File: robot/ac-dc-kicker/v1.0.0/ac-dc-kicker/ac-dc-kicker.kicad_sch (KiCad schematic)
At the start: 9 parts

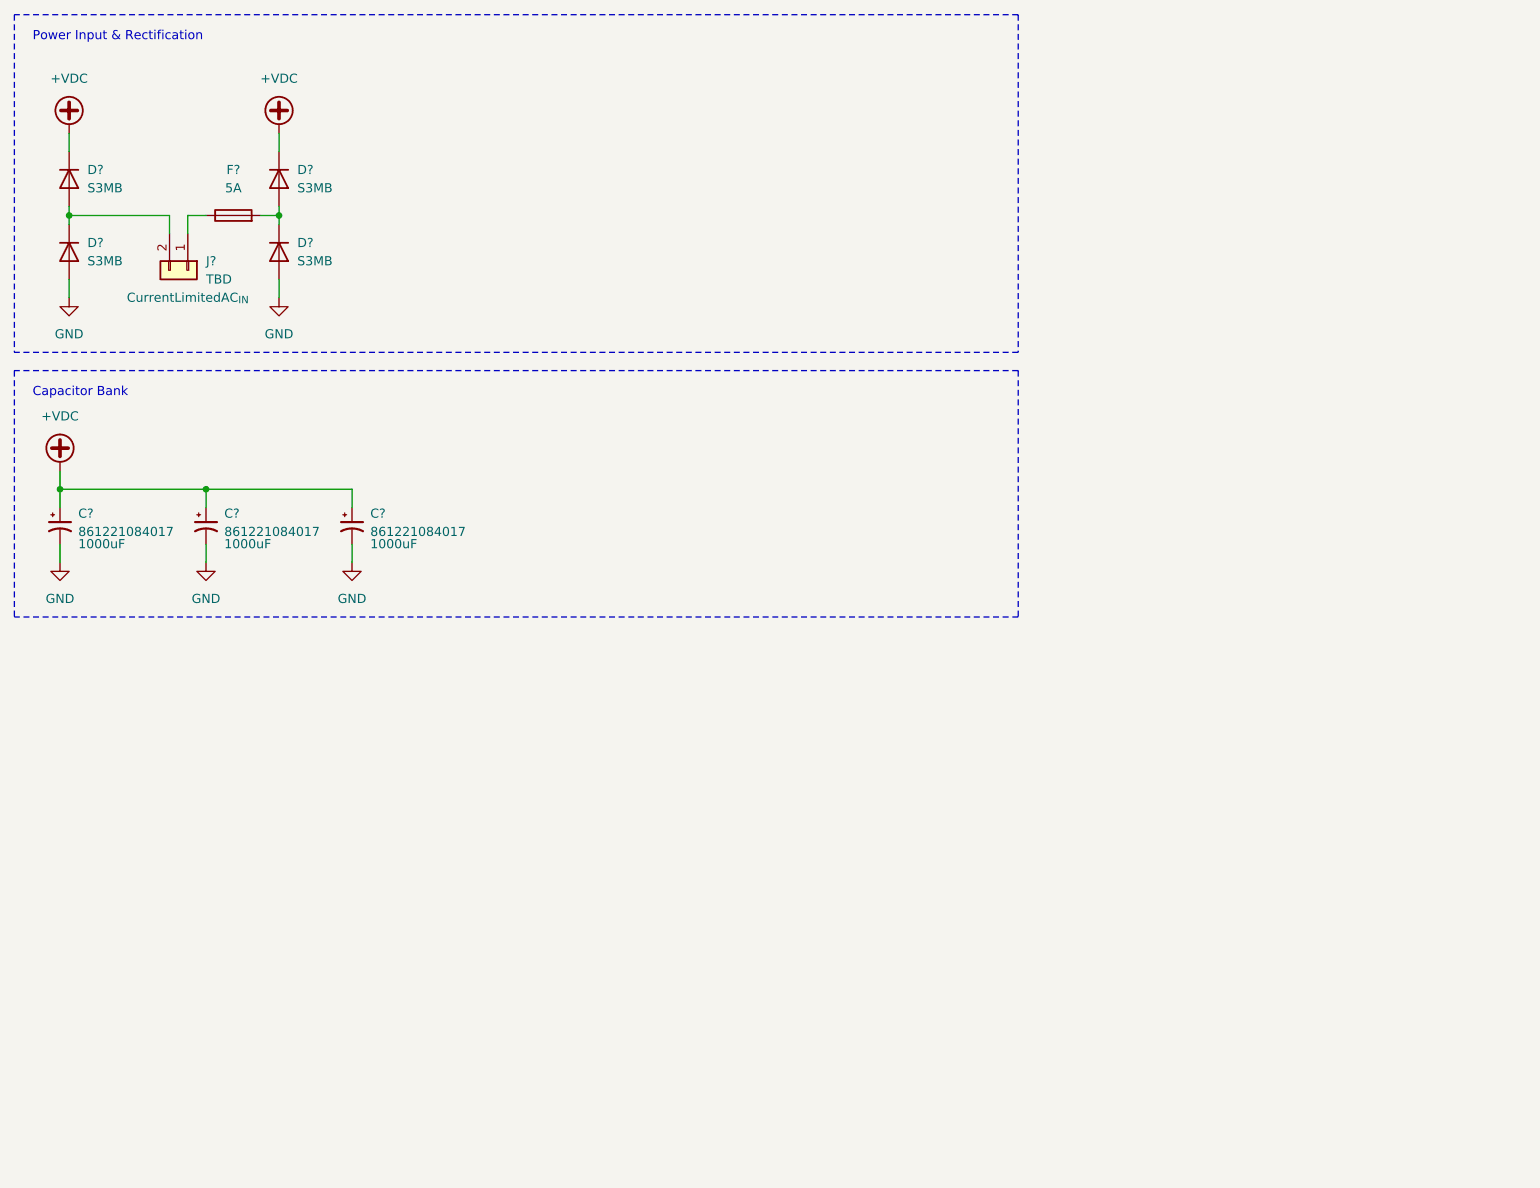
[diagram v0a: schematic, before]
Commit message: Bodge Bot Kicker
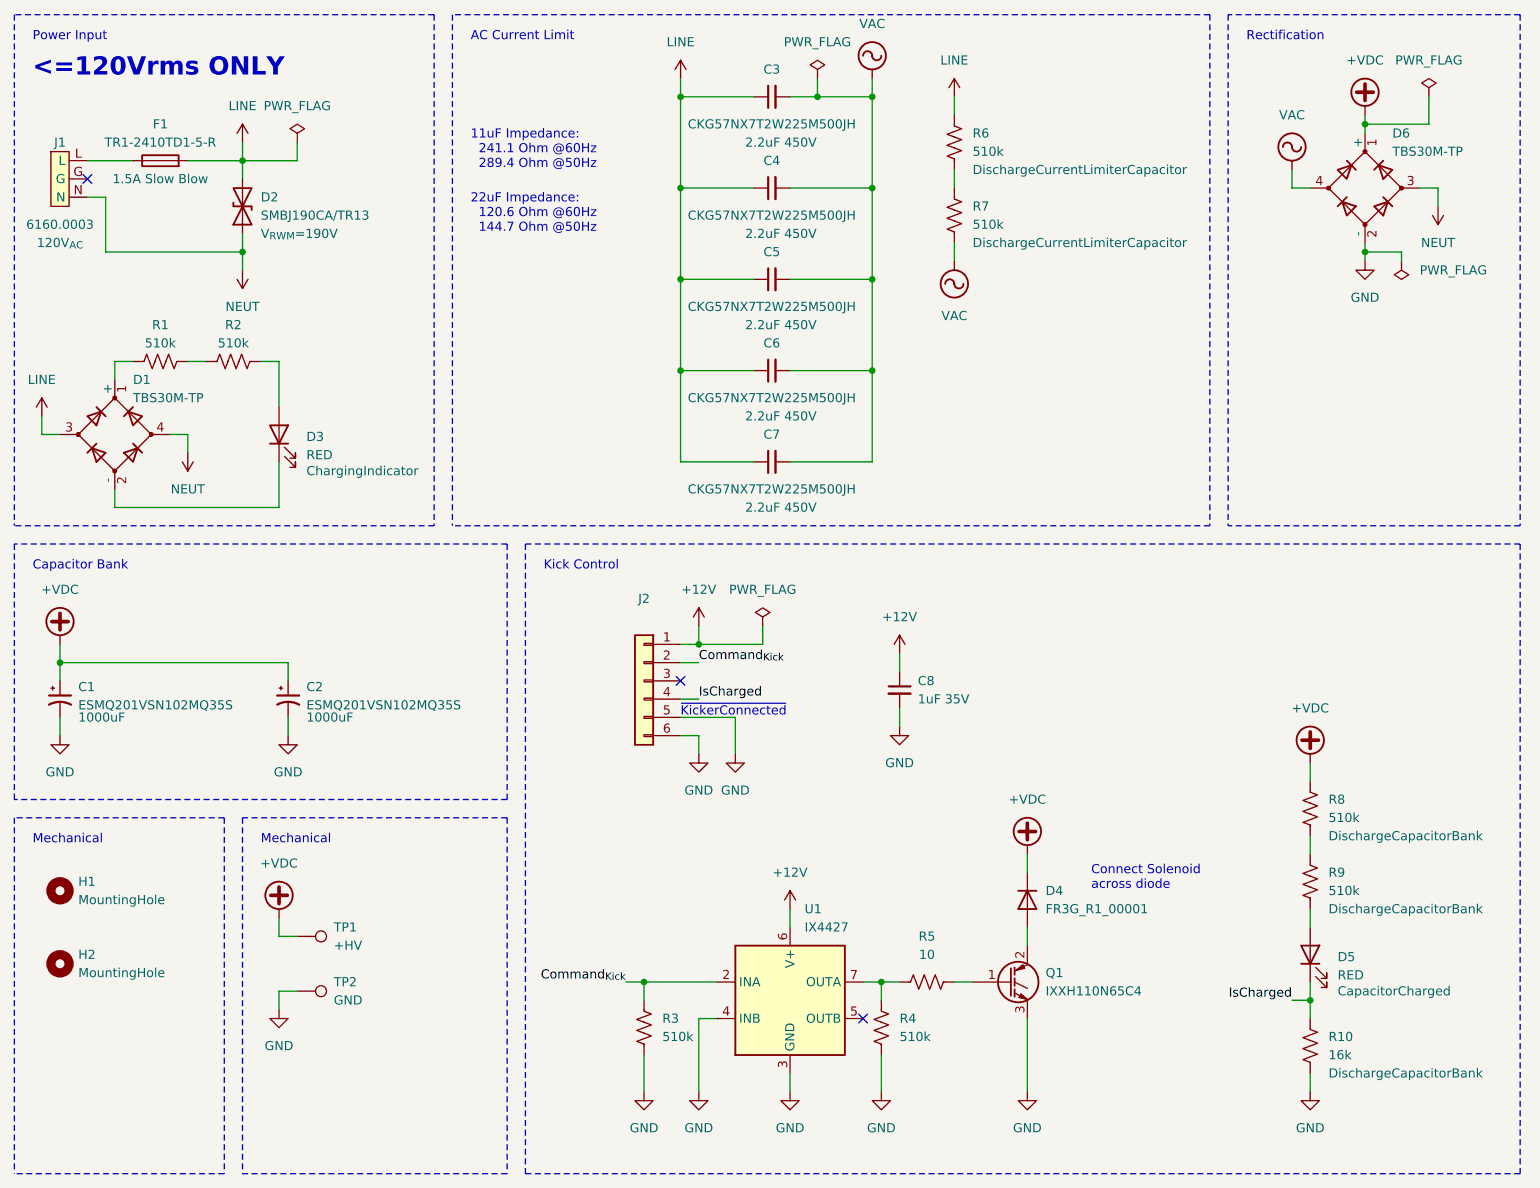
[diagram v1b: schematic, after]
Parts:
- removed C? (x2): 861221084017, symbol Device:C_Polarized_Small_US
- removed D? (x4): S3MB, symbol Device:D
- removed J?: TBD, symbol Connector_Generic:Conn_01x02
- added C2: ESMQ201VSN102MQ35S, AT-Capacitors:CP_Radial_D25.40mm_P10.00mm, symbol Device:C_Polarized_Small_US
- added C3, C4, C5, C6, C7: CKG57NX7T2W225M500JH, AT-Capacitors:CKG57N, symbol Device:C_Small
- added C8: 1uF 35V, LED_SMD:LED_0603_1608Metric, symbol Device:C_Small
- added D1, D6: TBS30M-TP, AT-IC:TBS, symbol Device:D_Bridge_+-AA
- added D2: SMBJ190CA/TR13, AT-Discrete:D_SMB_Non-Polar, symbol Device:D_TVS
- added D3, D5: RED, LED_SMD:LED_0603_1608Metric, symbol Device:LED
- added D4: FR3G_R1_00001, Diode_SMD:D_SMC, symbol Device:D
- added H1, H2: MountingHole, MountingHole:MountingHole_3.2mm_M3, symbol Mechanical:MountingHole
- added J1: 6160.0003, AT-Connectors:6160.0003, symbol AT-Connectors:Conn_ACPowerEntry_LGN
- added J2: ~, AT-Connectors:1x06_P2.5mm_ID0.8mm_OD2mm_TH, symbol Connector_Generic:Conn_01x06
- added Q1: IXXH110N65C4, Package_TO_SOT_THT:TO-247-3_Vertical, symbol Device:Q_NIGBT_GCE
- added R1, R2, R3, R4, R6, R7, R8, R9: 510k, Resistor_SMD:R_0805_2012Metric, symbol Device:R_US
- added R10: 16k, Resistor_SMD:R_0805_2012Metric, symbol Device:R_US
- added R5: 10, Resistor_SMD:R_0603_1608Metric, symbol Device:R_US
- added TP1: +HV, TestPoint:TestPoint_THTPad_D2.0mm_Drill1.0mm, symbol Connector:TestPoint
- added TP2: GND, TestPoint:TestPoint_THTPad_D2.0mm_Drill1.0mm, symbol Connector:TestPoint
- added U1: IX4427, Package_SO:SOIC-8_3.9x4.9mm_P1.27mm, symbol AT-PowerIC:IX4427
- C1: renamed from C?; value 861221084017 -> ESMQ201VSN102MQ35S; footprint (none) -> AT-Capacitors:CP_Radial_D25.40mm_P10.00mm
- F1: renamed from F?; value 5A -> TR1-2410TD1-5-R; footprint AT-Fuses:3557-2 -> AT-Fuses:Fuse_2410_6125Metric; Value2 (none) -> 1.5A Slow Blow
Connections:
- net +VDC: now also C2.1, D4.1 (K), D6.1 (+), R8.1, TP1.1
- net GND: now also C2.2, C8.2, D6.2 (-), J2.5 (Pin_5), J2.6 (Pin_6), Q1.3 (E), R10.2, R3.2, R4.2, TP2.1, U1.3 (GND), U1.4 (INB)
- net LINE: now reaches F1.2
- net LINE: now also C3.1, C4.1, C5.1, C6.1, C7.1, D1.3, D2.2 (A2), R6.1
- net at F1.1: now also J1.L
- new net: R6.2, R7.1
- new net: D1.1 (+), R1.1
- new net: R1.2, R2.1
- new net: Q1.1 (G), R5.2
- new net: D4.2 (A), Q1.2 (C)
- new net: D1.2 (-), D3.1 (K)
- new net: D3.2 (A), R2.2
- new net: R4.1, R5.1, U1.7 (OUTA)
- new net: R8.2, R9.1
- new net: D5.2 (A), R9.2
- new net +12V: C8.1, J2.1 (Pin_1), U1.6 (V+)
- new net Command_{Kick}: J2.2 (Pin_2), R3.1, U1.2 (INA)
- new net IsCharged: D5.1 (K), J2.4 (Pin_4), R10.1
- new net NEUT: D1.4, D2.1 (A1), D6.3, J1.N
- new net VAC: C3.2, C4.2, C5.2, C6.2, C7.2, D6.4, R7.2
- no-connect marks 0 -> 3
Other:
- note added: "11uF Impedance: 241.1 Ohm @60Hz 289.4 Ohm @50Hz"
- note added: "22uF Impedance: 120.6 Ohm @60Hz 144.7 Ohm @50Hz"
- note added: "<=120Vrms ONLY"
- note added: "AC Current Limit"
- note added: "Connect Solenoid across diode"
- note added: "Kick Control"
- note added: "Mechanical"
- note added: "Power Input"
- note added: "Rectification"
- note added: "~{KickerConnected}"
- note removed: "Power Input & Rectification"
- moved on the sheet: C1, F1
